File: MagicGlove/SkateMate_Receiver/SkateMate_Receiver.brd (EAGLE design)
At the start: 39.6 x 19.4 mm, 20 parts, among them IC1 LM1117IMPX-3.3, U1 ATMEGA328P-AU

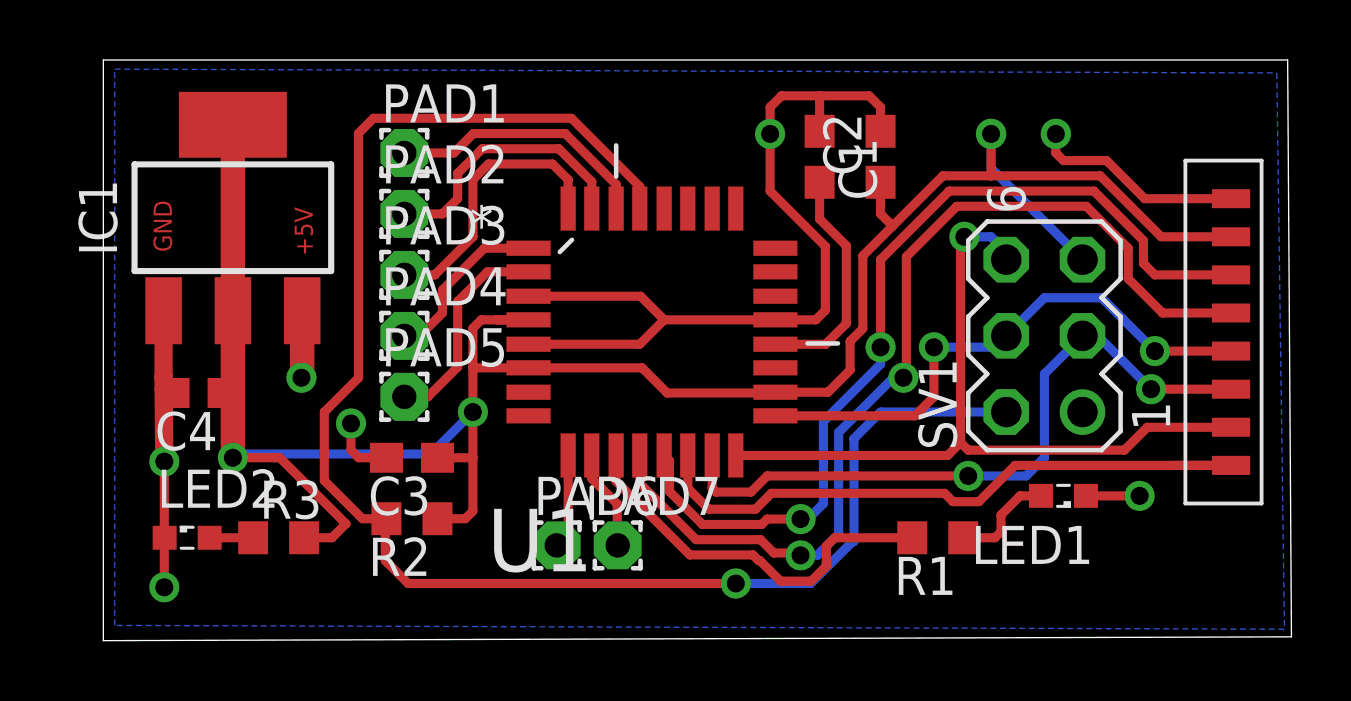
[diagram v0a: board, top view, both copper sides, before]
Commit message: Receiver Board v1.0 working
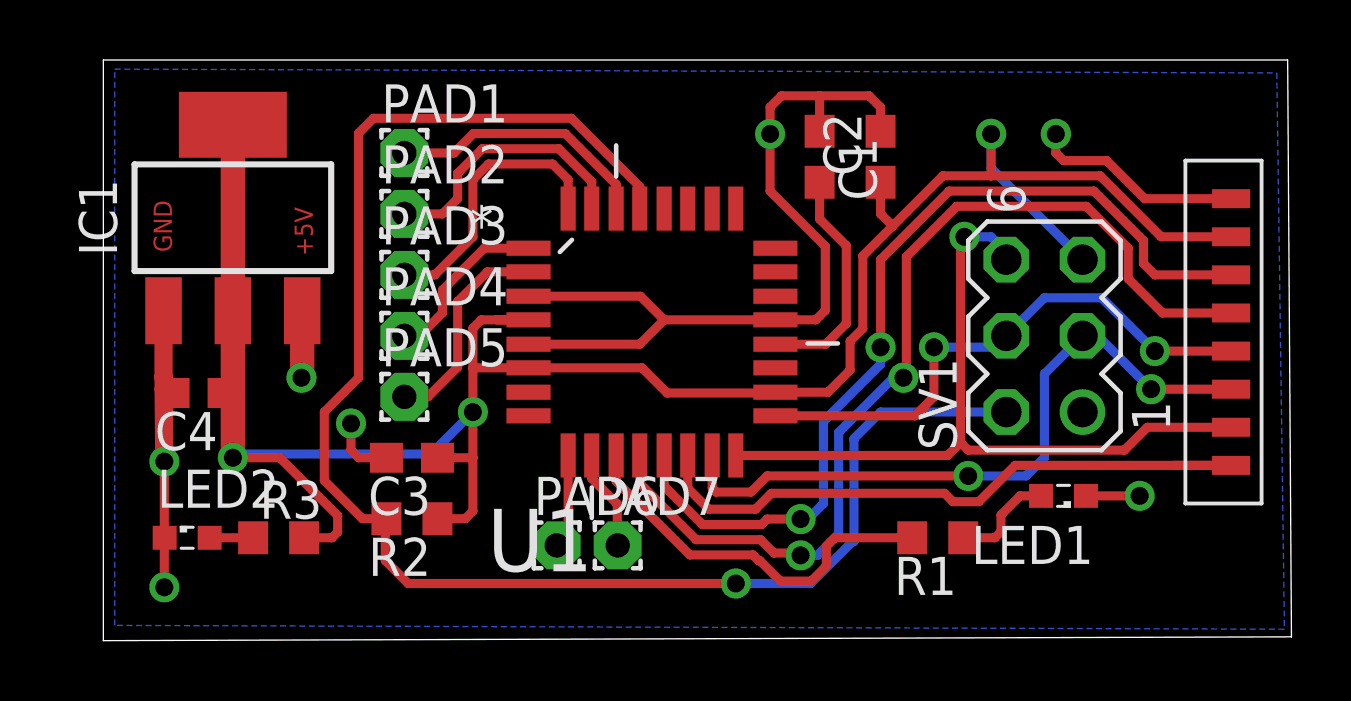
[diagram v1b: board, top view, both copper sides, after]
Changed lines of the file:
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@@
 <wire x1="28.194" y1="14.986" x2="33.02" y2="14.986" width="0.3048" layer="1"/>
 <wire x1="19.969875" y1="3.8735" x2="21.94735" y2="3.8735" width="0.3048" layer="1"/>
-<wire x1="18.6944" y1="6.1722" x2="18.8722" y2="5.9944" width="0.3048" layer="1"/>
 <wire x1="21.94735" y1="3.8735" x2="22.1263375" y2="4.0524875" width="0.3048" layer="1"/>
 <wire x1="22.1263375" y1="4.0524875" x2="23.241" y2="4.0524875" width="0.3048" layer="1"/>
-<wire x1="18.8722" y1="5.9944" x2="18.8722" y2="4.971175" width="0.3048" layer="1"/>
-<wire x1="18.8722" y1="4.971175" x2="19.969875" y2="3.8735" width="0.3048" layer="1"/>
+<wire x1="18.9738" y1="4.869575" x2="18.8722" y2="4.971175" width="0.3048" layer="1"/>
 <via x="23.241" y="4.0524875" extent="1-16" drill="0.6" diameter="0.4064"/>
+<wire x1="18.9738" y1="4.869575" x2="19.969875" y2="3.8735" width="0.3048" layer="1"/>
 <wire x1="23.241" y1="4.0524875" x2="23.4834875" y2="4.0524875" width="0.3048" layer="16"/>
 <wire x1="23.4834875" y1="4.0524875" x2="24.003" y2="4.572" width="0.3048" layer="16"/>
 <wire x1="25.908" y1="9.779" x2="25.908" y2="12.7" width="0.3048" layer="1"/>
 <wire x1="25.908" y1="12.7" x2="28.194" y2="14.986" width="0.3048" layer="1"/>
+<wire x1="18.6944" y1="6.1722" x2="18.6944" y2="5.148975" width="0.3048" layer="1"/>
+<wire x1="18.6944" y1="5.148975" x2="18.9738" y2="4.869575" width="0.3048" layer="1"/>
 </signal>
 <signal name="CSN">
@@
 <wire x1="4.318" y1="17.196" x2="4.318" y2="10.998" width="0.8128" layer="1"/>
 <contactref element="R3" pad="2"/>
+<wire x1="5.885575" y1="6.096" x2="4.318" y2="6.096" width="0.3048" layer="1"/>
 <wire x1="6.692" y1="3.429" x2="7.62" y2="3.429" width="0.3048" layer="1"/>
-<wire x1="8.0862875" y1="3.8952875" x2="7.62" y2="3.429" width="0.3048" layer="1"/>
-<wire x1="4.318" y1="6.096" x2="5.715" y2="6.096" width="0.3048" layer="1"/>
-<wire x1="5.715" y1="6.096" x2="5.885575" y2="6.096" width="0.3048" layer="1"/>
-<wire x1="5.885575" y1="6.096" x2="8.0862875" y2="3.8952875" width="0.3048" layer="1"/>
+<wire x1="7.62" y1="3.429" x2="7.8105" y2="3.6195" width="0.3048" layer="1"/>
+<wire x1="7.8105" y1="3.6195" x2="7.8105" y2="4.171075" width="0.3048" layer="1"/>
+<wire x1="7.8105" y1="4.171075" x2="5.885575" y2="6.096" width="0.3048" layer="1"/>
 </signal>
 <signal name="IRQ">
